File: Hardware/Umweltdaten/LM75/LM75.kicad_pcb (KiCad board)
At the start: 2 copper layers, 18 x 15 mm, 9 parts, among them IC2 LM75, P1 I2C

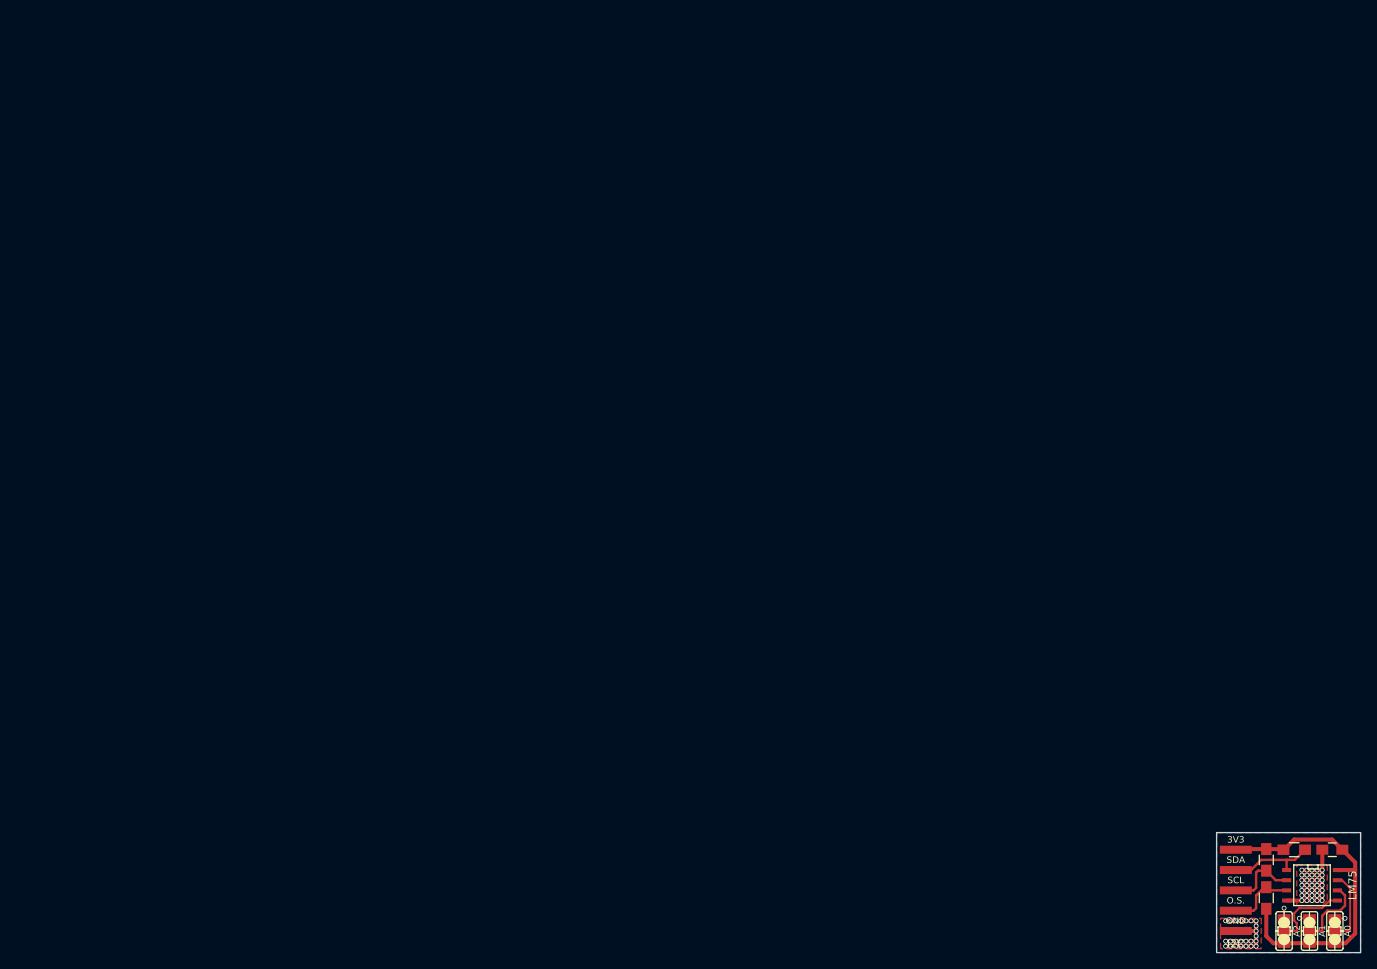
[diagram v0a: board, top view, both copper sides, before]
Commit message: create Gerber files
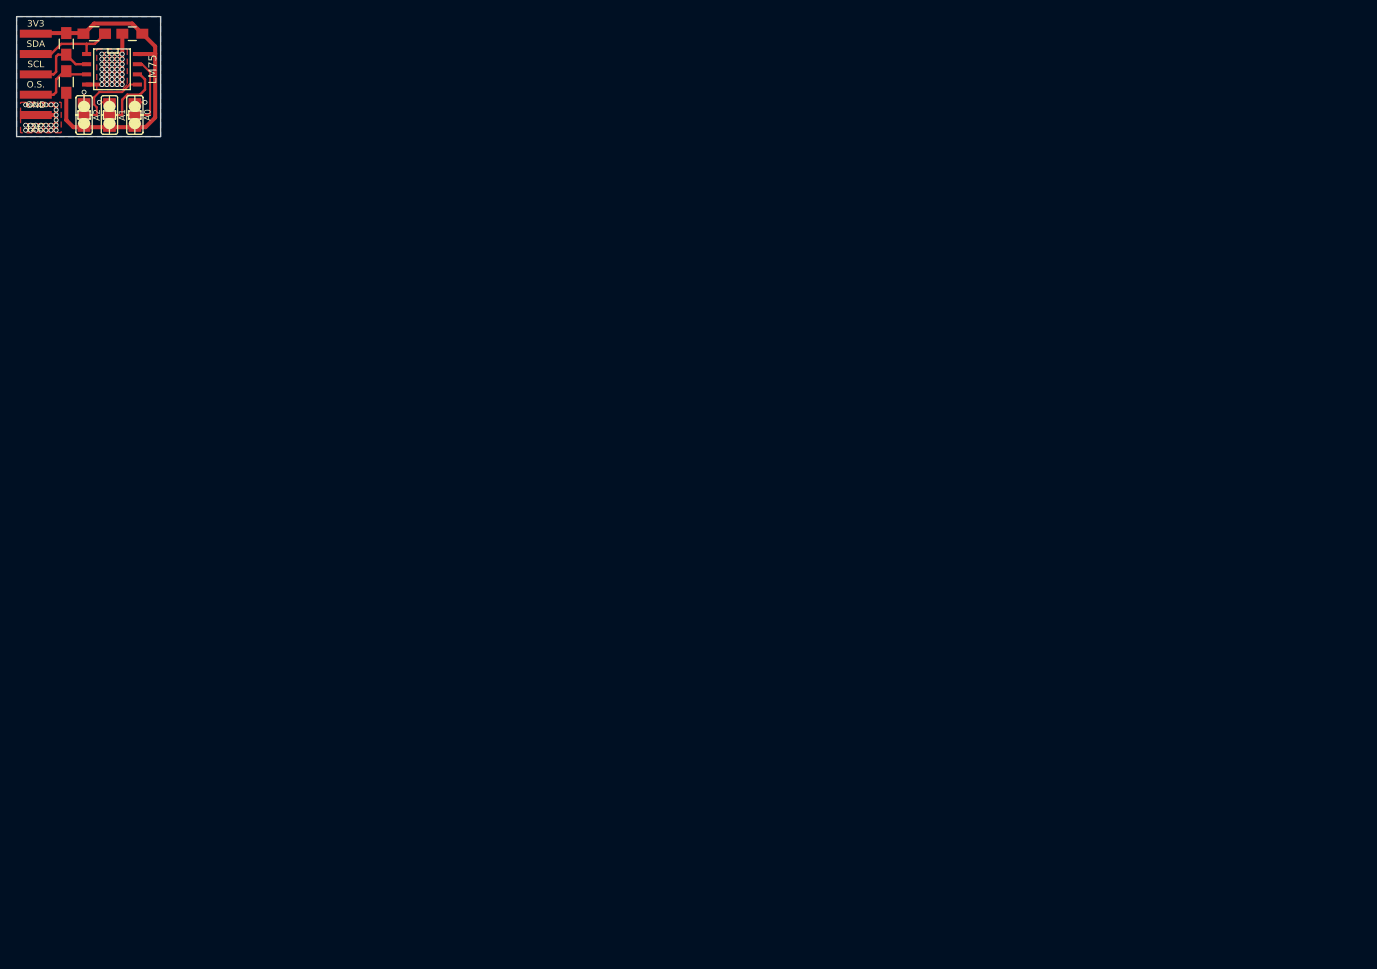
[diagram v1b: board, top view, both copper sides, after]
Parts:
- moved C1 181.4 mm to (14.5, 2.14)
- moved IC2 181.4 mm to (11.9, 6.58)
- moved JP1 181.4 mm to (14.8, 12.3)
- moved JP2 181.4 mm to (11.6, 12.3)
- moved JP3 181.4 mm to (8.43, 12.3)
- moved P1 181.4 mm to (2.40, 2.14)
- moved R1 181.4 mm to (6.21, 8.17)
- moved R2 181.4 mm to (6.21, 3.41)
- moved R3 181.4 mm to (9.70, 2.14)
